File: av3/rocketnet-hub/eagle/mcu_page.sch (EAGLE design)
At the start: 340 parts, among them J1 ROCKETBUS, J2 ROCKETBUS, J3 ROCKETBUS, J4 ROCKETBUS, J5 ROCKETBUS, J6 ROCKETBUS, J7 ROCKETBUS, J8 ROCKETBUS, J9 DEBUG-CONNECTOR, Q1 25MHz, U1 STM32F407V100-PIN_QFP, X1 87758-0416, X2 87758-0416, X3 87758-0416, X4 87758-0416, X5 87758-0416, X6 87758-0416, X7 87758-0416

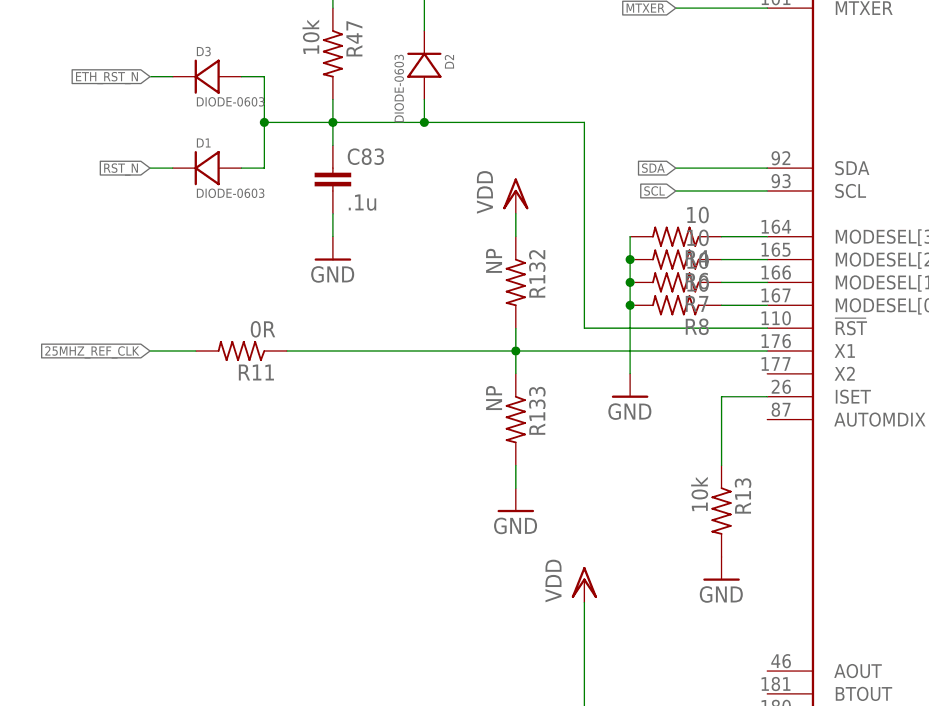
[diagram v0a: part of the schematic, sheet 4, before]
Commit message: added center mounting hole
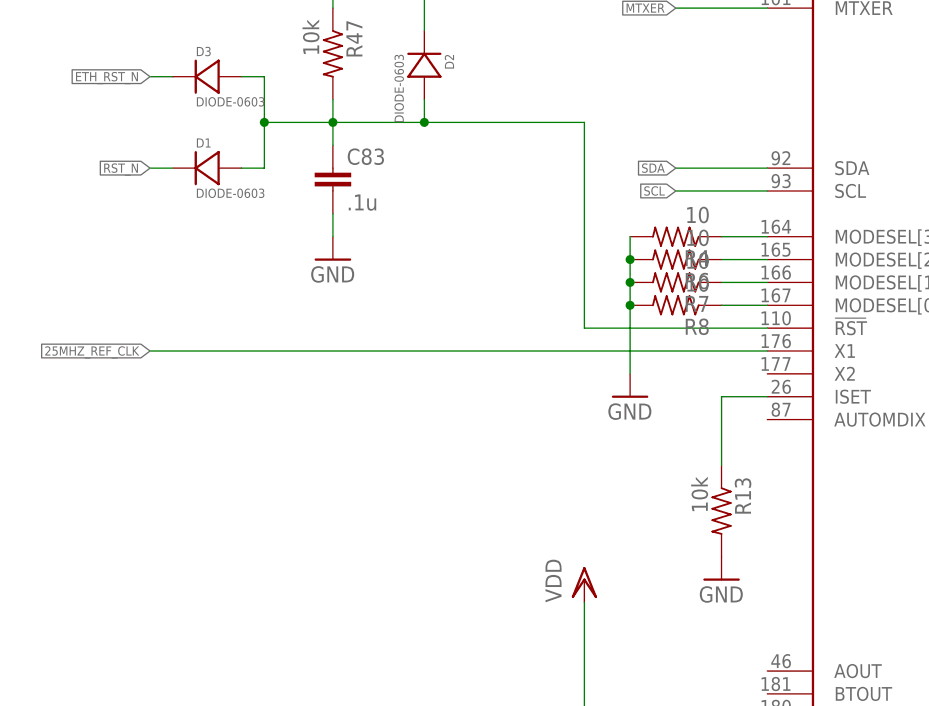
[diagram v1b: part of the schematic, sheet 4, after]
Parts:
- removed R11: 0R, rcl:R-US_R0402
- removed R132, R133: NP, rcl:R-US_R0402
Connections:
- removed net N$138: R11.1, R132.2, R133.1, U$14.X1
- net 25MHZ_REF_CLK: now also U$14.X1; no longer R11.2
- net GND: no longer R133.2
- net VDD: no longer R132.1
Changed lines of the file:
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@@
 <part name="TP28" library="testpad" deviceset="TP" device="TP06R"/>
 <part name="GND7" library="supply1" deviceset="GND" device=""/>
-<part name="R11" library="rcl" deviceset="R-US_" device="R0402" value="0R"/>
-<part name="VDD14" library="supply1" deviceset="VDD" device=""/>
-<part name="GND10" library="supply1" deviceset="GND" device=""/>
 <part name="R15" library="rcl" deviceset="R-US_" device="R0402" value="2.2k"/>
 <part name="R17" library="rcl" deviceset="R-US_" device="R0402" value="2.2k"/>
@@
 <part name="R131" library="rcl" deviceset="R-US_" device="R0402" value="10k"/>
 <part name="GND57" library="supply1" deviceset="GND" device=""/>
-<part name="R132" library="rcl" deviceset="R-US_" device="R0402" value="NP"/>
-<part name="R133" library="rcl" deviceset="R-US_" device="R0402" value="NP"/>
 <part name="C7" library="rcl" deviceset="C-EU" device="C0402"/>
 <part name="C35" library="rcl" deviceset="C-EU" device="C0402"/>
@@
 <instance part="R14" gate="G$1" x="195.58" y="30.48" rot="R90"/>
 <instance part="GND7" gate="1" x="187.96" y="236.22"/>
-<instance part="R11" gate="G$1" x="20.32" y="149.86" rot="R180"/>
-<instance part="VDD14" gate="G$1" x="50.8" y="167.64"/>
-<instance part="GND10" gate="1" x="50.8" y="132.08"/>
 <instance part="D3" gate="G$1" x="15.24" y="180.34"/>
 <instance part="R116" gate="G$1" x="66.04" y="86.36" rot="R180"/>
@@
 <instance part="R120" gate="G$1" x="66.04" y="27.94" rot="R180"/>
 <instance part="FRAME4" gate="G$1" x="287.02" y="7.62"/>
-<instance part="R132" gate="G$1" x="50.8" y="157.48" rot="R270"/>
-<instance part="R133" gate="G$1" x="50.8" y="142.24" rot="R270"/>
 </instances>
 <busses>
@@
 <wire x1="187.96" y1="241.3" x2="187.96" y2="238.76" width="0.1524" layer="91"/>
 </segment>
-<segment>
-<pinref part="GND10" gate="1" pin="GND"/>
-<pinref part="R133" gate="G$1" pin="2"/>
-<wire x1="50.8" y1="134.62" x2="50.8" y2="137.16" width="0.1524" layer="91"/>
-</segment>
 </net>
 <net name="+3V3" class="1">
@@
 <net name="25MHZ_REF_CLK" class="0">
 <segment>
-<pinref part="R11" gate="G$1" pin="2"/>
-<wire x1="10.16" y1="149.86" x2="15.24" y2="149.86" width="0.1524" layer="91"/>
 <label x="10.16" y="149.86" size="1.016" layer="95" rot="R180" xref="yes"/>
+<pinref part="U$14" gate="G$1" pin="X1"/>
+<wire x1="10.16" y1="149.86" x2="78.74" y2="149.86" width="0.1524" layer="91"/>
 </segment>
 </net>
@@
 <wire x1="48.26" y1="223.52" x2="50.8" y2="223.52" width="0.1524" layer="91"/>
 </segment>
-<segment>
-<pinref part="VDD14" gate="G$1" pin="VDD"/>
-<wire x1="50.8" y1="162.56" x2="50.8" y2="165.1" width="0.1524" layer="91"/>
-<pinref part="R132" gate="G$1" pin="1"/>
-</segment>
 </net>
 <net name="ETH_EN" class="0">
@@
 </segment>
 </net>
-<net name="N$138" class="0">
-<segment>
-<pinref part="R11" gate="G$1" pin="1"/>
-<pinref part="U$14" gate="G$1" pin="X1"/>
-<wire x1="25.4" y1="149.86" x2="50.8" y2="149.86" width="0.1524" layer="91"/>
-<pinref part="R133" gate="G$1" pin="1"/>
-<wire x1="50.8" y1="149.86" x2="78.74" y2="149.86" width="0.1524" layer="91"/>
-<wire x1="50.8" y1="147.32" x2="50.8" y2="149.86" width="0.1524" layer="91"/>
-<junction x="50.8" y="149.86"/>
-<pinref part="R132" gate="G$1" pin="2"/>
-<wire x1="50.8" y1="149.86" x2="50.8" y2="152.4" width="0.1524" layer="91"/>
-</segment>
-</net>
